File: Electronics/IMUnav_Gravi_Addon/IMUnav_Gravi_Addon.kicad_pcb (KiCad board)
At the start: 2 copper layers, 45 x 42 mm, 6 parts, among them J1 Conn_01x03_Pin, J2 Conn_01x03_Pin, J3 Conn_02x08_Odd_Even, J4 Conn_01x03_Socket, J5 BMP280-module, U1 MT3608-module

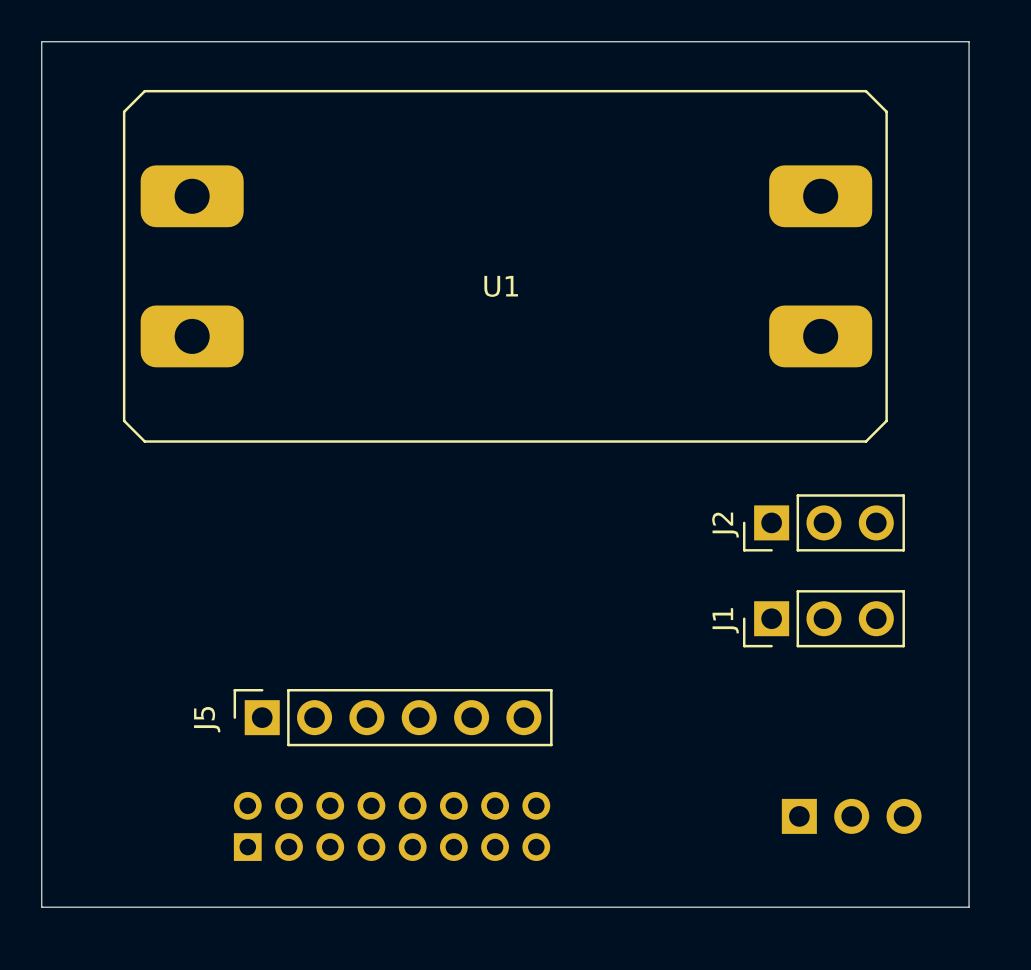
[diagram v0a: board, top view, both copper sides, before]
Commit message: addon pcb routing
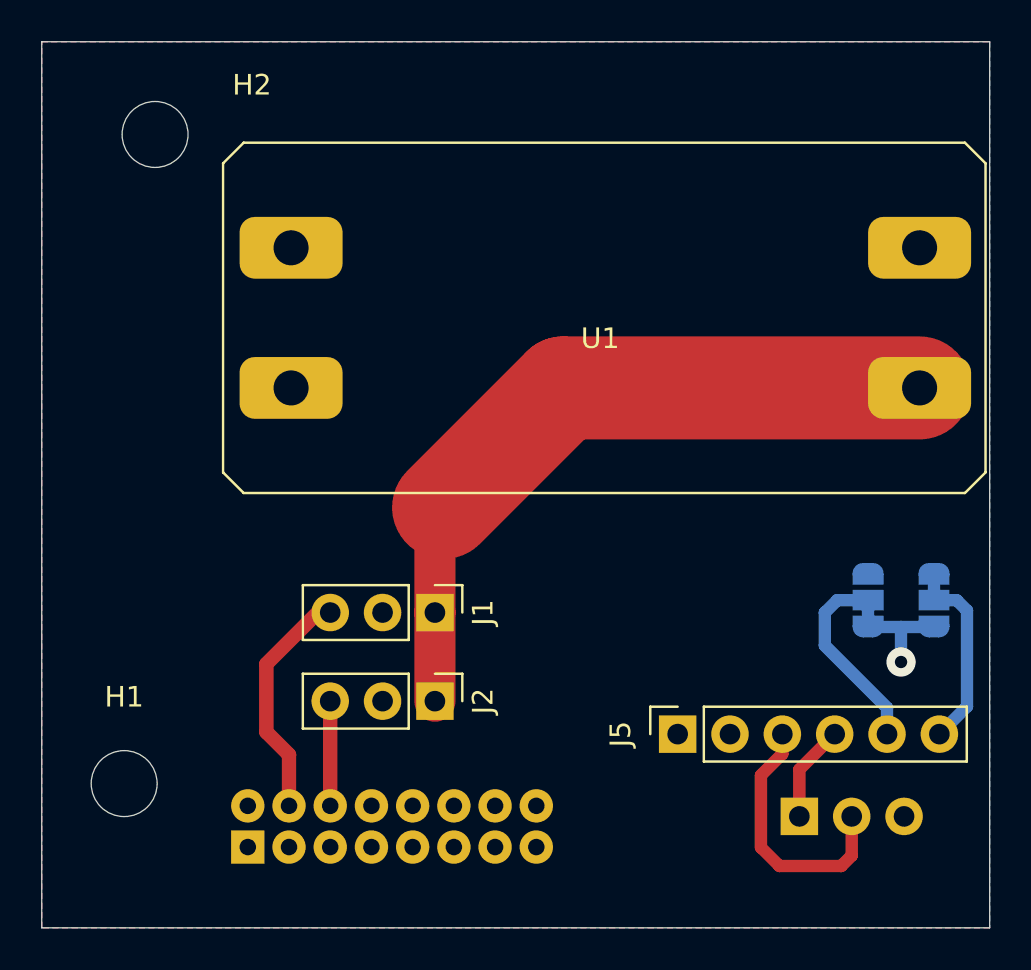
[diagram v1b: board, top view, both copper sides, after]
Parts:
- added H1: MountingHole, MountingHole:MountingHole_3.2mm_M3, F.Cu at (4.00, 36.0)
- added H2: MountingHole, MountingHole:MountingHole_3.2mm_M3, F.Cu at (5.50, 4.50)
- added JP1: SolderJumper_3_Bridged12, Jumper:SolderJumper-3_P1.3mm_Bridged12_RoundedPad1.0x1.5mm_NumberLabels, B.Cu at (43.3, 27.1)
- added JP2: SolderJumper_3_Bridged12, Jumper:SolderJumper-3_P1.3mm_Bridged12_RoundedPad1.0x1.5mm_NumberLabels, B.Cu at (40.1, 27.1)
- moved J5 20.2 mm to (30.9, 33.6)
- moved J2 18.5 mm to (19.1, 32.0), turned to -90 degrees
- moved J1 16.3 mm to (19.1, 27.7), turned to -90 degrees
- moved U1 5.41 mm to (27.1, 13.9)
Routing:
- net Vdrive: track 0.00 -> 35.8 mm
- net SCL: track 0.00 -> 12.8 mm
- net SERVO1: track 0.00 -> 11.5 mm
- net CSB: track 0.00 -> 10.0 mm
- net SDO: track 0.00 -> 8.36 mm
- net SERVO2: track 0.00 -> 5.08 mm
- net +3V3: track 0.00 -> 4.90 mm, vias 0 -> 1
- net SDA: track 0.00 -> 4.70 mm
- added copper zone on F.Cu, net +3V3
- added copper zone on B.Cu, net GND
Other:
- board size 45 x 42 mm -> 46 x 43 mm
